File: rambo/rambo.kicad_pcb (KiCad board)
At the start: 2 copper layers, 130.9 x 81.3 mm, 43 parts, among them J1 Barrel_Jack_Switch, J2 USB_B, J3 Conn_02x25_Odd_Even, Q1 2N7000, SW1 SW_DIP_x04, U1 74LS139, U10 74HCT04, U11 74LS245, U12 74HCT00, U13 74LS85, U14 74HCT02, U15 74LS139, U2 74HCT273, U3 74LS191, U4 74LS191, U5 74LS191, U6 74LS191, U7 74LS191, U8 AS6C4008-55PCN, U9 AS6C4008-55PCN

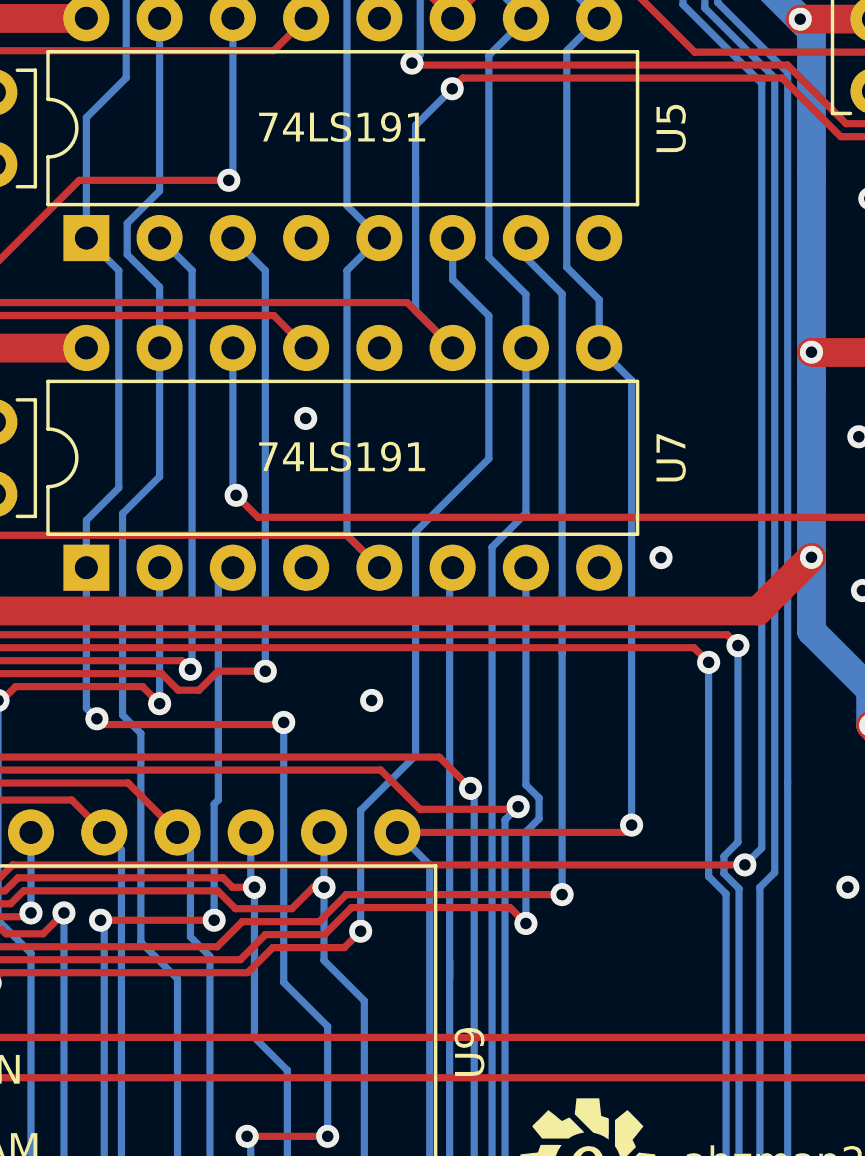
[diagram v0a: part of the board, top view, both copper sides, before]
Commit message: fixed erc and drc
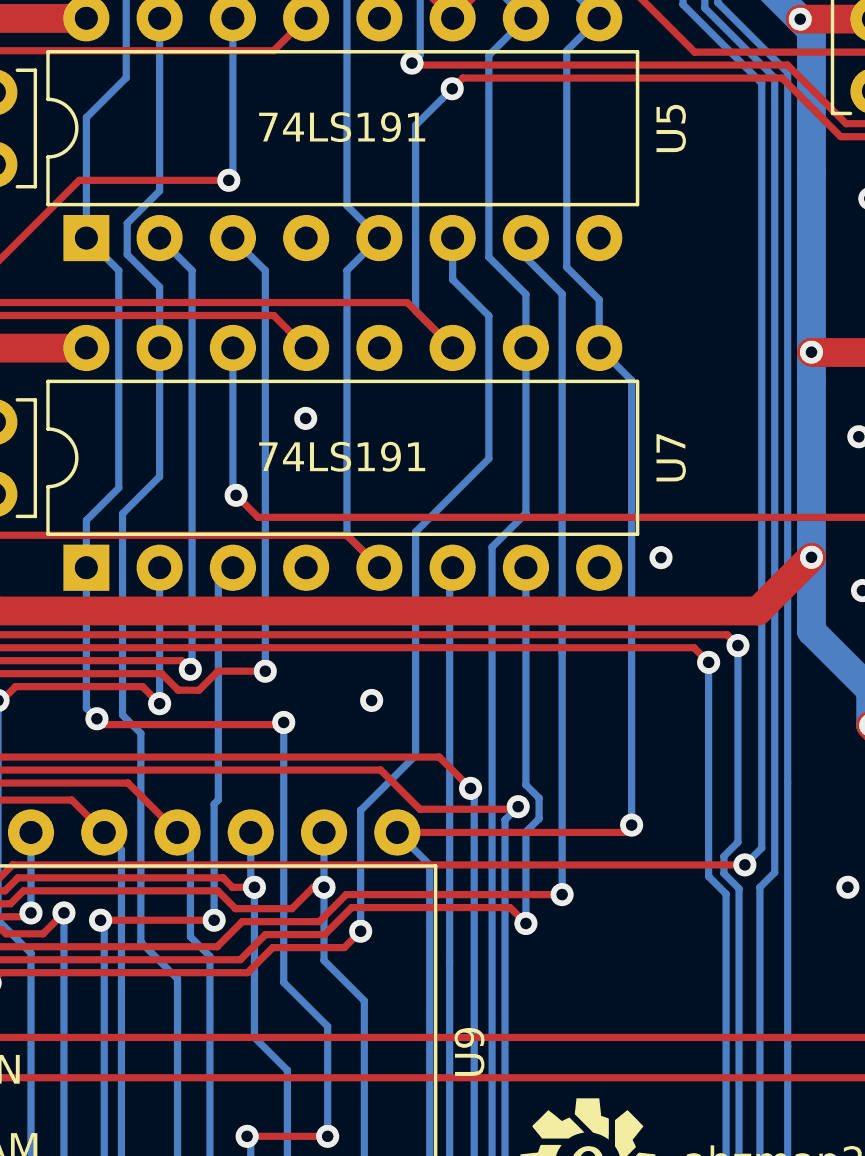
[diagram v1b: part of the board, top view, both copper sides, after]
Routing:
- net /~{AREGLWR}: track 80.0 -> 79.2 mm
- net /AR2: track 61.9 -> 61.3 mm
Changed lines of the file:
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@@
   (via (at 172.593 123.825) (size 0.8) (drill 0.4) (layers "F.Cu" "B.Cu") (net 26))
   (segment (start 154.323489 144.168489) (end 154.323489 128.378511) (width 0.25) (layer "B.Cu") (net 26))
-  (segment (start 172.503489 115.988489) (end 172.503489 116.593489) (width 0.25) (layer "B.Cu") (net 26))
   (segment (start 172.503489 123.735489) (end 172.593 123.825) (width 0.25) (layer "B.Cu") (net 26))
   (segment (start 155.448 127.254) (end 155.448 126.751) (width 0.25) (layer "B.Cu") (net 26))
@@
   (segment (start 243.961621 85.211621) (end 243.961621 81.403057) (width 0.25) (layer "F.Cu") (net 42))
   (segment (start 242.334644 79.77608) (end 231.648 79.77608) (width 0.25) (layer "F.Cu") (net 42))
-  (segment (start 243.512101 81.589255) (end 243.512101 87.302101) (width 0.25) (layer "F.Cu") (net 43))
   (segment (start 242.148446 80.2256) (end 243.512101 81.589255) (width 0.25) (layer "F.Cu") (net 43))
   (segment (start 243.512101 87.302101) (end 245.745 89.535) (width 0.25) (layer "F.Cu") (net 43))
+  (segment (start 243.512101 81.589255) (end 243.512101 87.302101) (width 0.25) (layer "F.Cu") (net 43))
   (segment (start 233.05 84.445) (end 233.05 81.1096) (width 0.25) (layer "F.Cu") (net 43))
   (segment (start 233.05 81.1096) (end 233.934 80.2256) (width 0.25) (layer "F.Cu") (net 43))
@@
   (segment (start 171.323 93.427) (end 171.323 89.535) (width 0.25) (layer "B.Cu") (net 58))
   (segment (start 171.323 89.535) (end 171.323 86.995) (width 0.25) (layer "B.Cu") (net 58))
-  (segment (start 171.323 89.535) (end 171.323 88.773) (width 0.25) (layer "B.Cu") (net 58))
   (segment (start 171.323 86.995) (end 172.593 85.725) (width 0.25) (layer "B.Cu") (net 58))
   (segment (start 172.608 94.712) (end 171.323 93.427) (width 0.25) (layer "B.Cu") (net 58))
